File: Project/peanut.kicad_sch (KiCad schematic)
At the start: 17 parts, among them J1 USB_C_Receptacle_USB2.0, SW2 SKQGABE010, U1 STM32F072C8Tx, U2 AP2112K-3.3, U3 PRTR5V0U2X

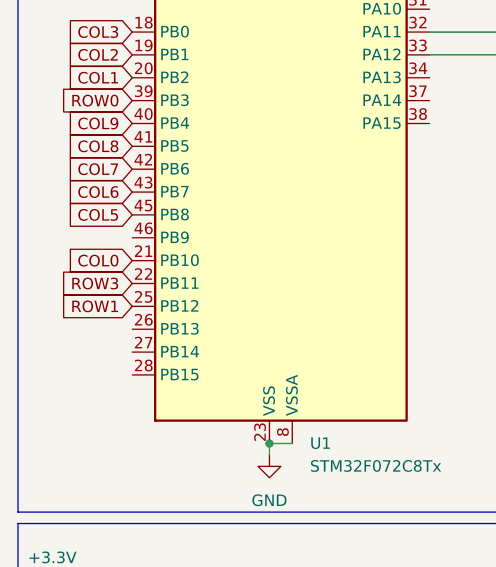
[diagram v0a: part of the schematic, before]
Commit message: firmware
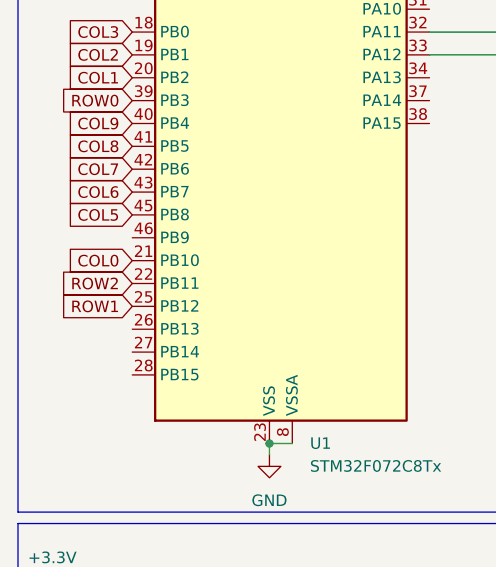
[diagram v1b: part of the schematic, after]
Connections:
- net ROW3 renamed ROW2
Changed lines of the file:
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@@
 		)
 	)
-	(global_label "ROW3"
+	(global_label "ROW2"
 		(shape input)
 		(at 31.75 87.63 180)
@@
 		)
 		(instances
-			(project "tsuru alice"
+			(project "peanut"
 				(path "/a7769bc2-6a19-42ef-91a1-19bc3a696dfe"
 					(page "2")
